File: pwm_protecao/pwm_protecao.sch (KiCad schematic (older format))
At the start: 28 parts, among them Q1 BC556, Q2 PN2222A, Q3 2N3904, Q4 2N3906, Q5 IRLZ44N, Q6 2N3904, Q7 2N3906, U1 4N25, U4 LF357, U5 NE555

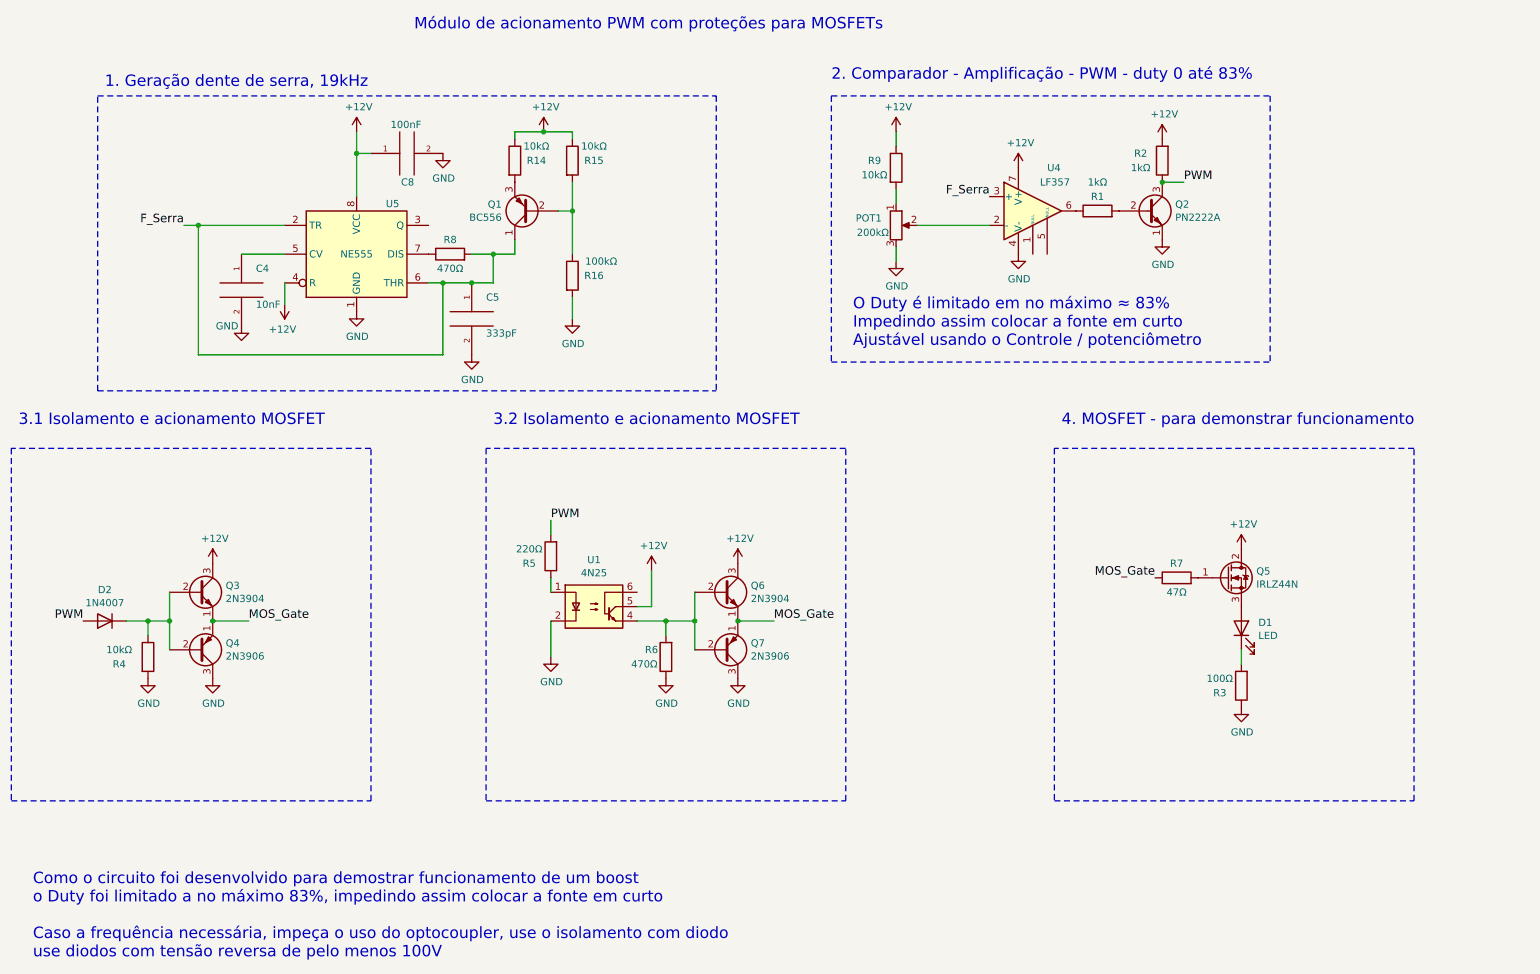
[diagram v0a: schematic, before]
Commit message: Up pcb
Signed-off-by: fgl27 <fglfgl27@gmail.com>
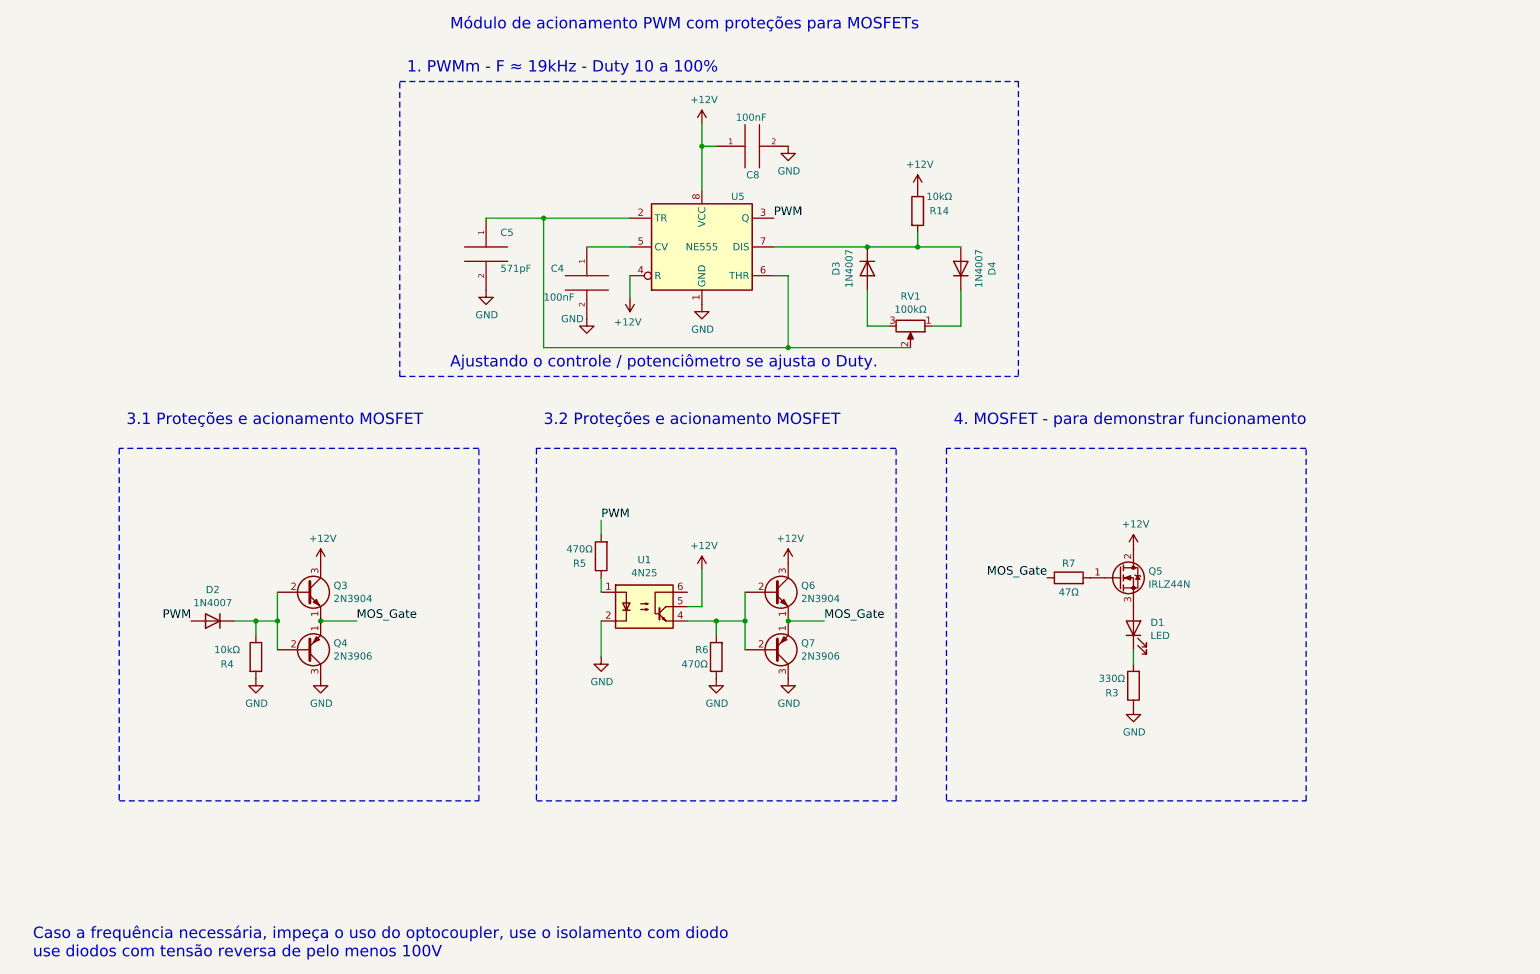
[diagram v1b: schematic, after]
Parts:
- removed POT1: 200kΩ, Potentiometer_THT:Potentiometer_Alps_RK163_Single_Horizontal, symbol Device:R_POT
- removed Q1: BC556, Package_TO_SOT_THT:TO-92_Wide, symbol Transistor_BJT:BC556
- removed Q2: PN2222A, Package_TO_SOT_THT:TO-92_Inline, symbol Transistor_BJT:PN2222A
- removed R1, R2: 1kΩ, Resistor_THT:R_Axial_DIN0207_L6.3mm_D2.5mm_P10.16mm_Horizontal, symbol Device:R
- removed R15, R9: 10kΩ, Resistor_THT:R_Axial_DIN0207_L6.3mm_D2.5mm_P10.16mm_Horizontal, symbol Device:R
- removed R16: 100kΩ, Resistor_THT:R_Axial_DIN0207_L6.3mm_D2.5mm_P10.16mm_Horizontal, symbol Device:R
- removed R8: 470Ω, Resistor_THT:R_Axial_DIN0207_L6.3mm_D2.5mm_P10.16mm_Horizontal, symbol Device:R
- removed U4: LF357, Package_DIP:DIP-8_W7.62mm_LongPads, symbol Amplifier_Operational:LF357
- added D3, D4: 1N4007, Diode_THT:D_DO-41_SOD81_P10.16mm_Horizontal, symbol Diode:1N4007
- added RV1: 100kΩ, Potentiometer_THT:Potentiometer_Alps_RK163_Single_Horizontal, symbol Device:R_POT
- C4: value 10nF -> 100nF
- C5: value 333pF -> 571pF
- R3: value 100Ω -> 330Ω
- R5: value 220Ω -> 470Ω
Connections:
- net PWM: now also U5.3 (Q)
- net at U5.7 (DIS): now also R14.2, D3.1 (K), D4.2 (A)
- net F_Serra: no longer names the net of C5.1, U5.2 (TR), U5.6 (THR)
- net F_Serra: now also RV1.2
- new net: D4.1 (K), RV1.1
- new net: D3.2 (A), RV1.3
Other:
- note added: "1. PWMm - F ≈ 19kHz - Duty 10 a 100%"
- note added: "3.1 Proteções e acionamento MOSFET"
- note added: "3.2 Proteções e acionamento MOSFET"
- note added: "Ajustando o controle / potenciômetro se ajusta o Duty."
- note added: "Caso a frequência necessária, impeça o uso do optocoupler, use o isolamento com diodo\nuse diodos com tensão reversa de pelo menos 100V"
- note removed: "1. Geração dente de serra, 19kHz"
- note removed: "2. Comparador - Amplificação - PWM - duty 0 até 83%"
- note removed: "3.1 Isolamento e acionamento MOSFET"
- note removed: "3.2 Isolamento e acionamento MOSFET"
- note removed: "Como o circuito foi desenvolvido para demostrar funcionamento de um boost\no Duty foi limitado a no máximo 83%, impedindo assim colocar a fonte em curto\n\nCaso a frequência necessária, impeça o uso do optocoupler, use o isolamento com diodo\nuse diodos com tensão reversa de pelo menos 100V"
- note removed: "O Duty é limitado em no máximo ≈ 83%\nImpedindo assim colocar a fonte em curto\nAjustável usando o Controle / potenciômetro"
- moved on the sheet: C4, C5, C8, D1, D2, Q3, Q4, Q5, Q6, Q7, R14, R3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
